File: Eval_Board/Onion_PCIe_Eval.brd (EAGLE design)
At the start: 70 x 60 mm, 7 parts, among them J1 61400416021, J2 7499010211A, J3 629722000214, Q1 LORA_MPCIE

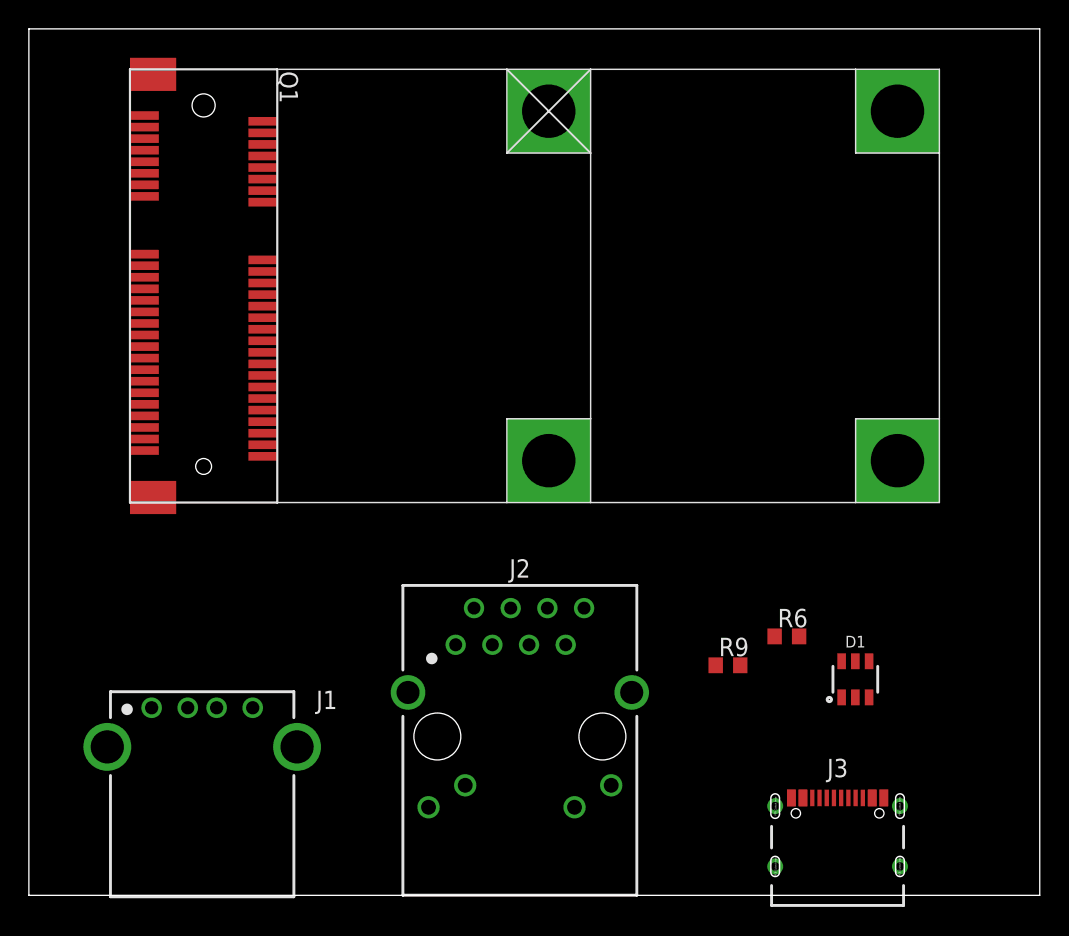
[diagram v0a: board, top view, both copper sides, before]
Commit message: - small changes to the sikscreen of the module - continued design of Eval Board
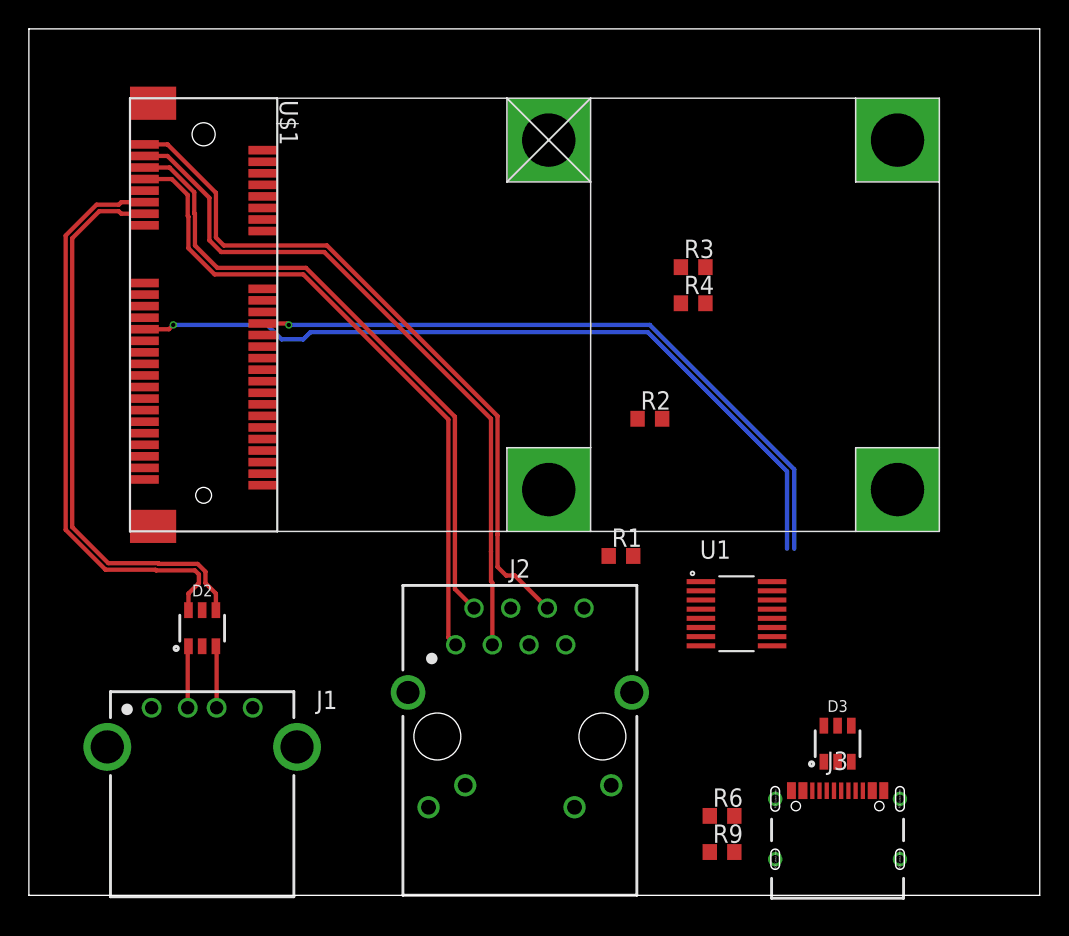
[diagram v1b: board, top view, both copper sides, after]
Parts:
- removed D1: 82400102 5V, Wurth_EMC Components_WE-TVS:WE-TVS_SOT23-6L
- removed Q1: LORA_MPCIE, Eigene-Rietig:MINI_PCIE_CONNECTOR_5.2H
- added D2, D3: 82400102 5V, Wurth_EMC Components_WE-TVS:WE-TVS_SOT23-6L
- added R1, R2, R3, R4: 5k1, rcl:R0603
- added U$1: ONION_OMEGA2S_MPCIE, Eigene-Rietig:MINI_PCIE_CONNECTOR_5.2H
- added U1: FT230XS, Eigene-Rietig:SSOP-16_FTD
- moved R6 13.2 mm to (48.0, 5.50)
- moved R9 12.9 mm to (48.0, 3.00)
- moved J3 0.50 mm to (56.0, 2.50)
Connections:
- new net CONSOLE_RXD: U$1.24, U1.1
- new net CONSOLE_TXD: U$1.25, U1.4
- new net ETH_RX_N: J2.3, R2.2, U$1.3
- new net ETH_RX_P: J2.6, R1.2, U$1.1
- new net ETH_TX_N: J2.1, R4.1, U$1.7
- new net ETH_TX_P: J2.2, R3.1, U$1.5
- new net N$1: R1.1, R2.1
- new net N$3: R3.2, R4.2
- new net N$4: U1.10, U1.11, U1.3
- new net USB_DN_N: D2.6, U$1.11
- new net USB_DN_P: D2.4, U$1.13
- new net USB_DN_PROT_N: D2.1, J1.2
- new net USB_DN_PROT_P: D2.3, J1.3
- net +5V: now also D2.5, D3.5, U1.12; no longer D1.5
- net GND: now also D2.2, D3.2, U$1.15, U$1.18, U$1.21, U$1.26, U$1.27, U$1.29, U$1.34, U$1.35, U$1.37, U$1.4, U$1.40, U$1.43, U$1.50, U$1.9, U1.13, U1.5; no longer D1.2
- net USB_D_N: now also D3.1; no longer D1.3
- net USB_D_P: now also D3.3; no longer D1.1
- net USB_D_PROT_N: now also D3.6, U1.8; no longer D1.4
- net USB_D_PROT_P: now also D3.4, U1.9; no longer D1.6
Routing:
- net CONSOLE_TXD: track 0.00 -> 54.6 mm, vias 0 -> 1
- net ETH_RX_P: track 0.00 -> 49.1 mm
- net ETH_RX_N: track 0.00 -> 49.0 mm
- net CONSOLE_RXD: track 0.00 -> 46.5 mm, vias 0 -> 1
- net ETH_TX_N: track 0.00 -> 45.9 mm
- net ETH_TX_P: track 0.00 -> 44.6 mm
- net USB_DN_N: track 0.00 -> 40.1 mm
- net USB_DN_P: track 0.00 -> 39.3 mm
- net USB_DN_PROT_P: track 0.00 -> 4.28 mm
- net USB_DN_PROT_N: track 0.00 -> 4.28 mm
